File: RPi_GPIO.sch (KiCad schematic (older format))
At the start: 1 part, among them J300 RPi_GPIO

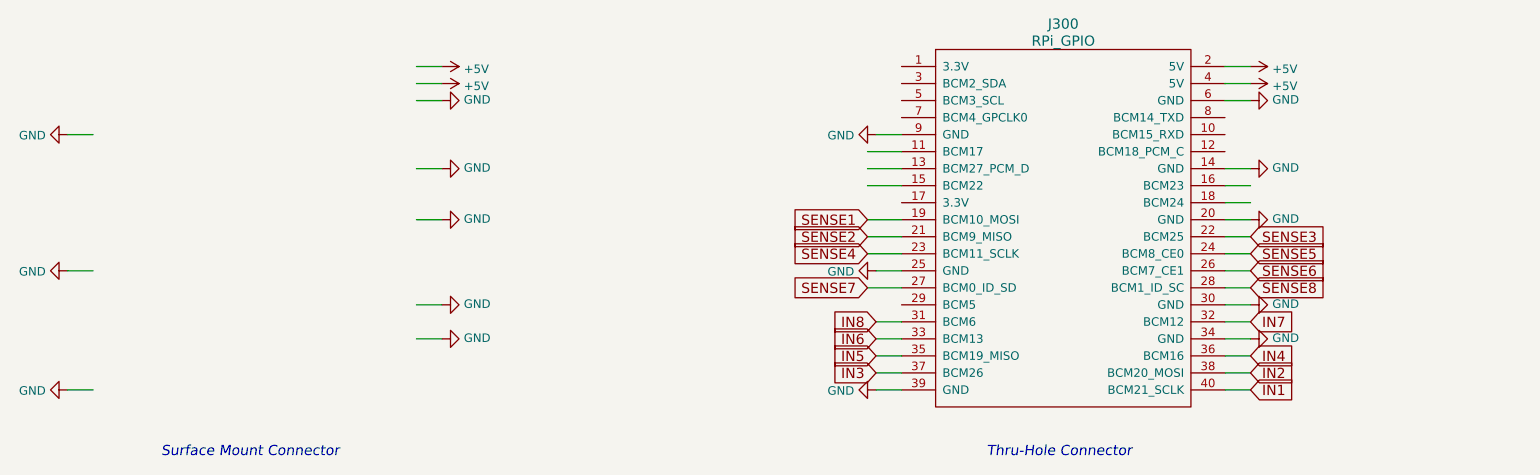
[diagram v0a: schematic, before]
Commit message: finished routing
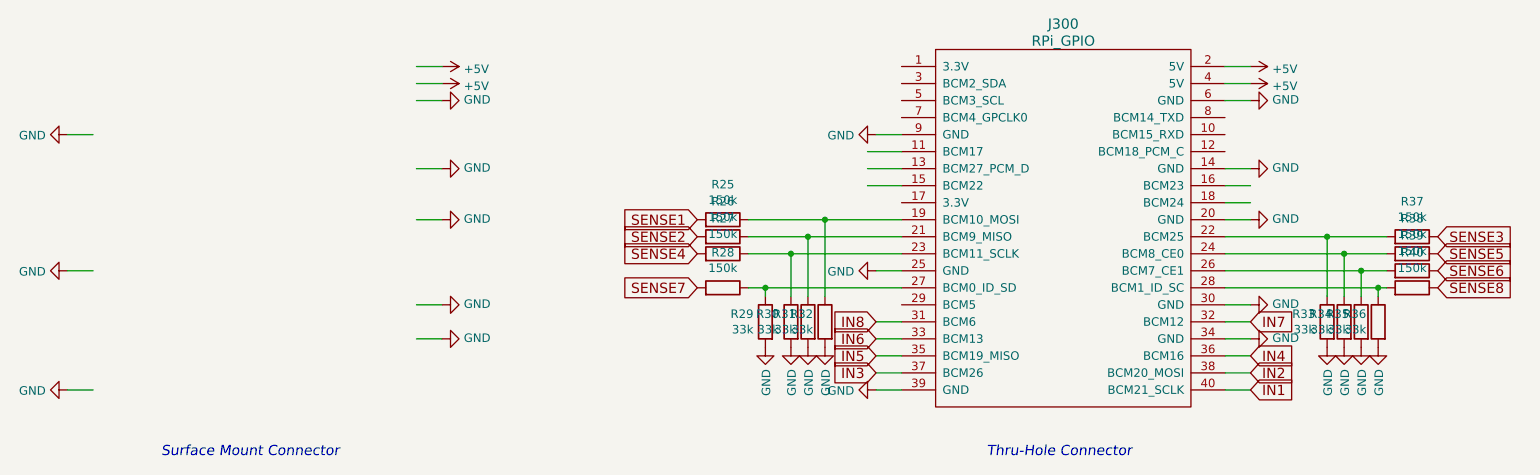
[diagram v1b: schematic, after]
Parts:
- added R25, R26, R27, R28, R37, R38, R39, R40: 150k, Resistors_SMD:R_0603, symbol R
- added R29, R30, R31, R32, R33, R34, R35, R36: 33k, Resistors_SMD:R_0603, symbol R
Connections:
- wire segments 41 -> 49

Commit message: final PCB as ordered
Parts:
- J300: LCSC P/N (none) -> C50982
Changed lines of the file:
@@
 F 2 "RPi_Hat:Pin_Header_Straight_2x20" H 7500 2700 60  0001 C CNN
 F 3 "" H 7500 2700 60  0000 C CNN
+F 4 "C50982" H 7500 2700 60  0001 C CNN "LCSC P/N"
 	1    7500 2700
 	1    0    0    -1
